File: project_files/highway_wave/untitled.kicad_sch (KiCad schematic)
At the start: 17 parts

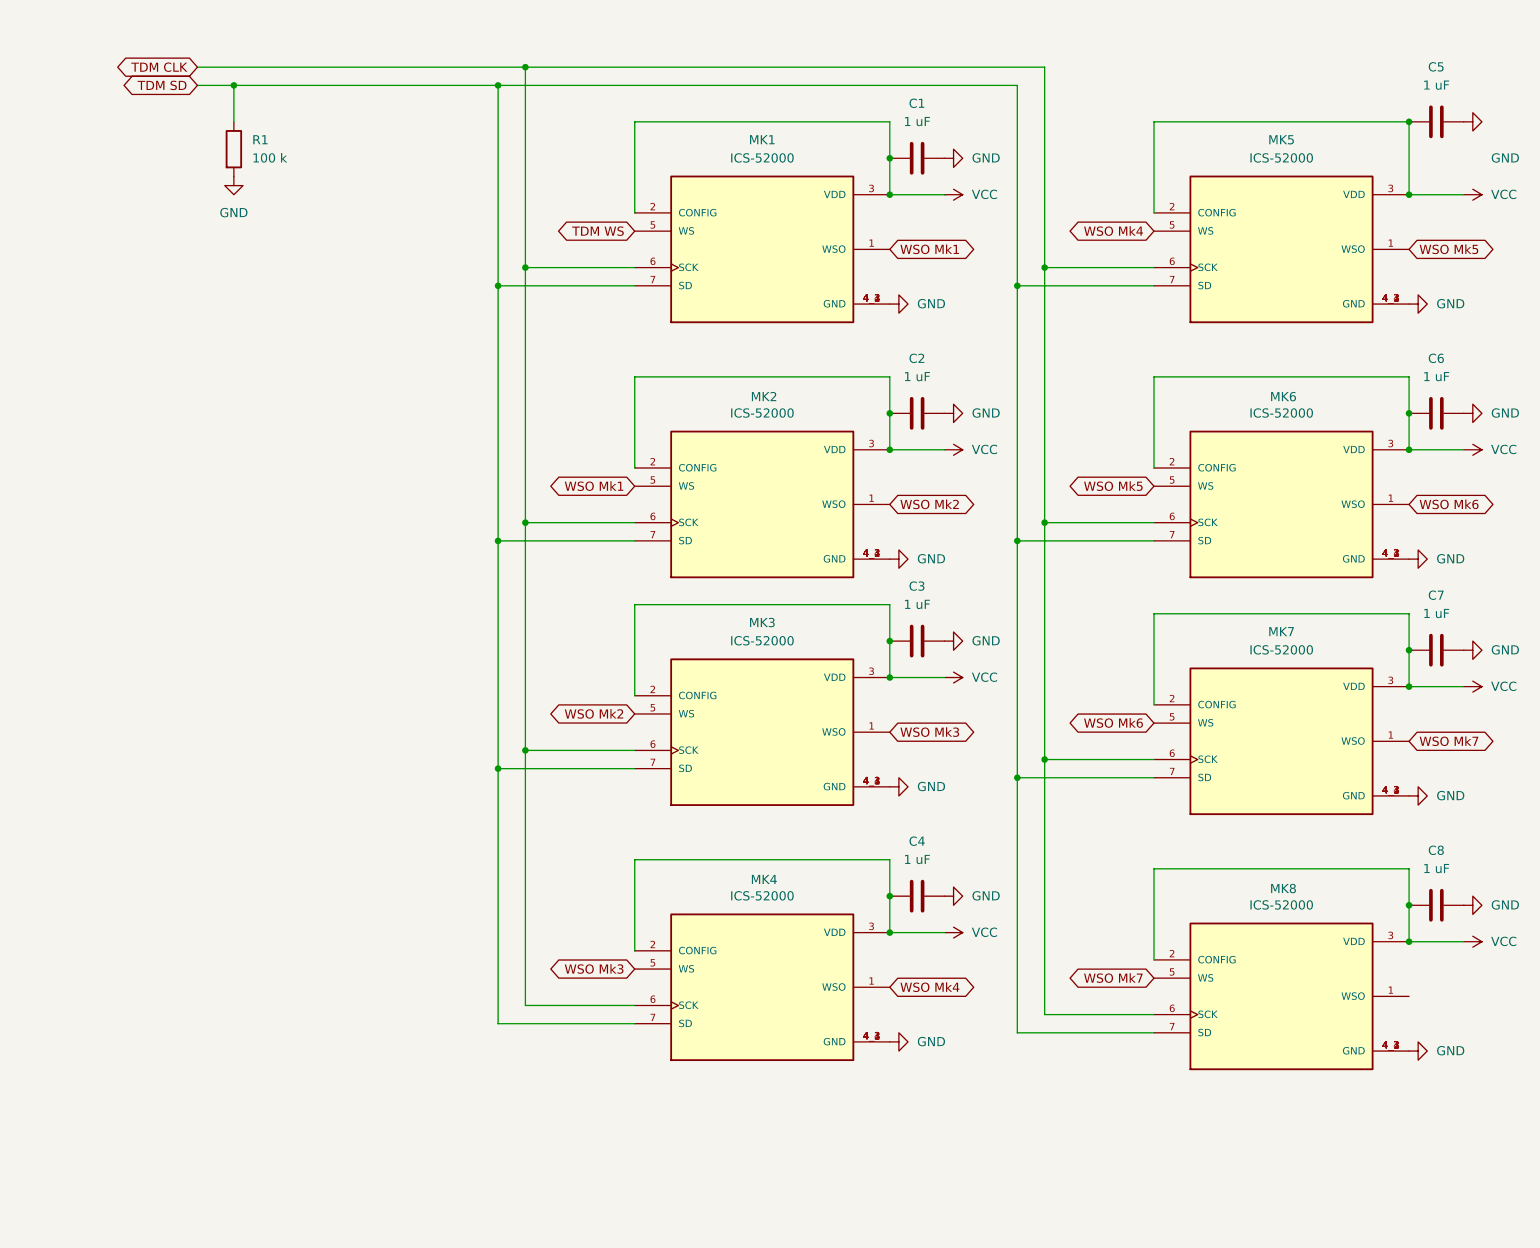
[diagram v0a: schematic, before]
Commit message: random committ
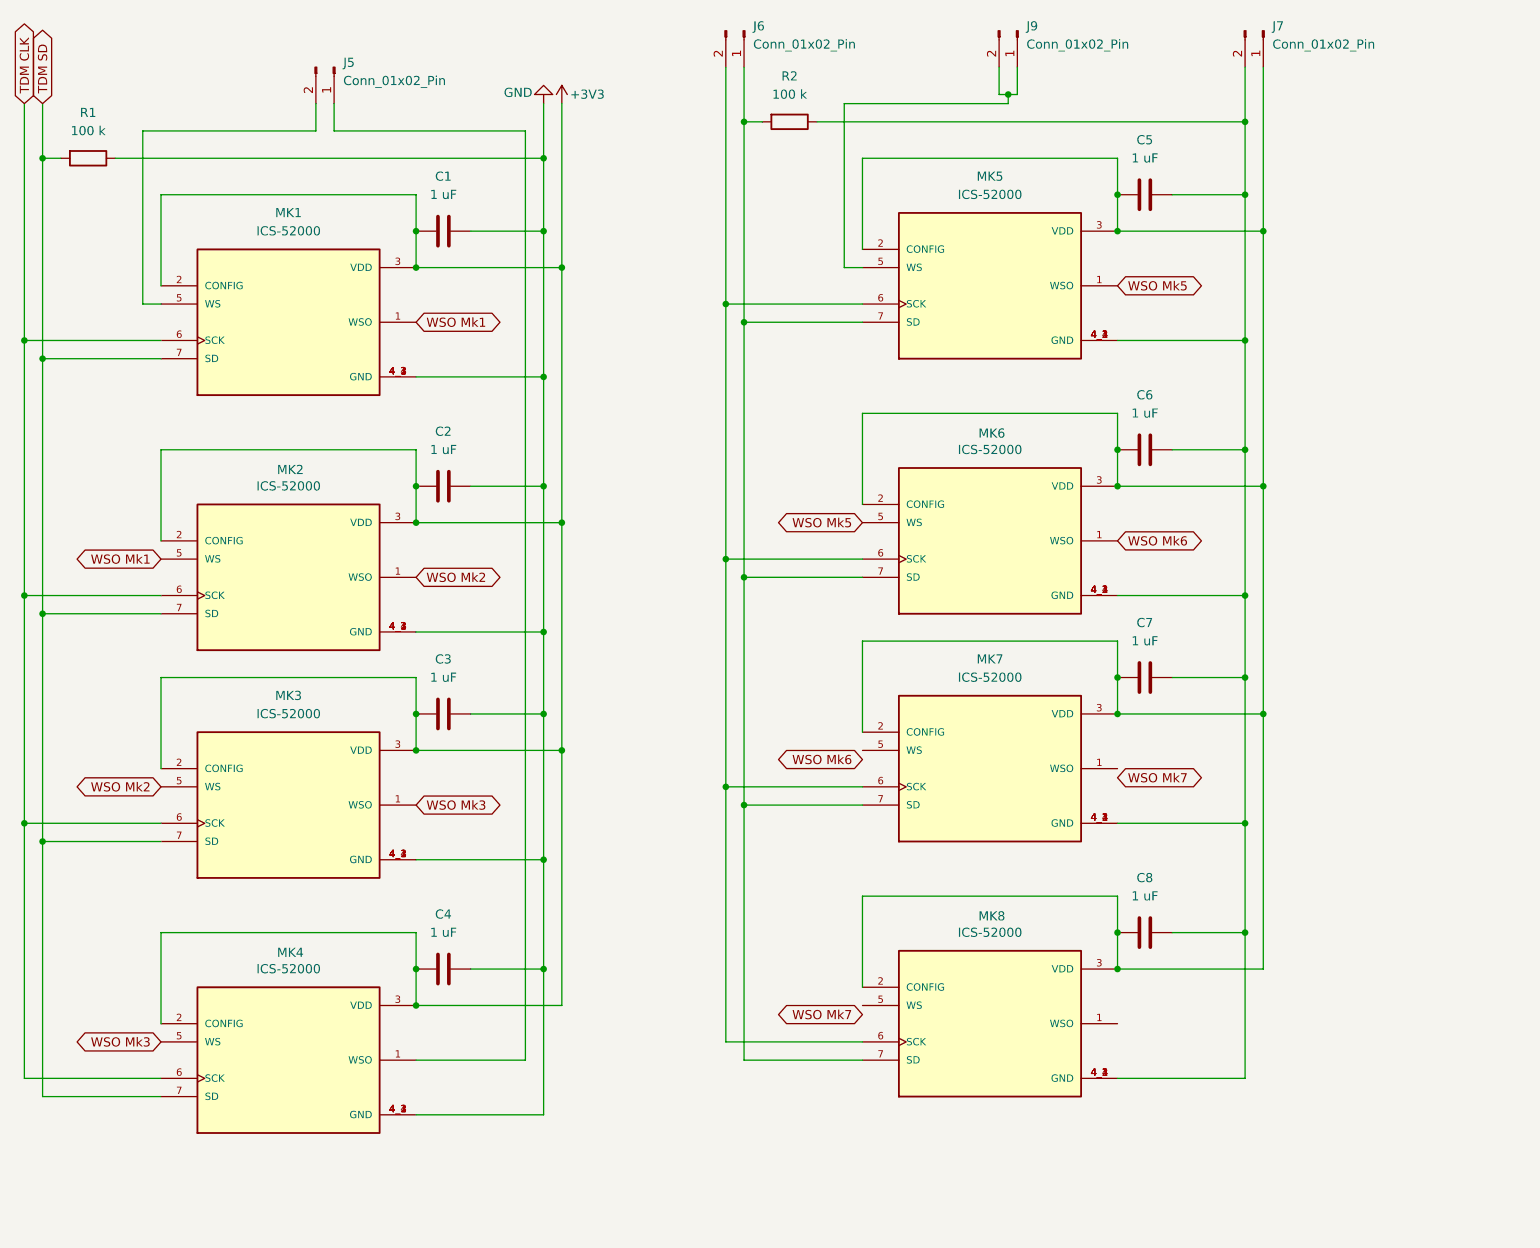
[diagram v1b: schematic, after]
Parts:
- added J5, J6, J7, J9: Conn_01x02_Pin, Connector_Phoenix_GMSTB:PhoenixContact_GMSTBVA_2,5_2-G_1x02_P7.50mm_Vertical, symbol Connector:Conn_01x02_Pin
- added R2: 100 k, Resistor_THT:R_Axial_DIN0207_L6.3mm_D2.5mm_P7.62mm_Horizontal, symbol Device:R
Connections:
- net GND: now also R1.1; no longer C5.2, C6.2, C7.2, C8.2, MK5.4_1 (GND), MK5.4_2 (GND), MK5.4_3 (GND), MK5.4_4 (GND), MK6.4_1 (GND), MK6.4_2 (GND), MK6.4_3 (GND), MK6.4_4 (GND), MK7.4_1 (GND), MK7.4_2 (GND), MK7.4_3 (GND), MK7.4_4 (GND), MK8.4_1 (GND), MK8.4_2 (GND), MK8.4_3 (GND), MK8.4_4 (GND), R1.2
- net TDM CLK: no longer MK5.6 (SCK), MK6.6 (SCK), MK7.6 (SCK), MK8.6 (SCK)
- net TDM SD: now also R1.2; no longer MK5.7 (SD), MK6.7 (SD), MK7.7 (SD), MK8.7 (SD), R1.1
- net WSO Mk6: no longer MK7.5 (WS)
- net WSO Mk7: no longer MK7.1 (WSO), MK8.5 (WS)
- net TDM WS: no longer names the net of MK1.5 (WS)
- net TDM WS: now also J5.2 (Pin_2)
- net VCC: no longer names the net of C5.1, C6.1, C7.1, C8.1, MK5.2 (CONFIG), MK5.3 (VDD), MK6.2 (CONFIG), MK6.3 (VDD), MK7.2 (CONFIG), MK7.3 (VDD), MK8.2 (CONFIG), MK8.3 (VDD)
- net VCC: now also J7.1 (Pin_1); no longer C1.1, C2.1, C3.1, C4.1, MK1.2 (CONFIG), MK1.3 (VDD), MK2.2 (CONFIG), MK2.3 (VDD), MK3.2 (CONFIG), MK3.3 (VDD), MK4.2 (CONFIG), MK4.3 (VDD)
- net WSO Mk4: no longer names the net of MK5.5 (WS)
- net WSO Mk4: now also J9.1 (Pin_1), J9.2 (Pin_2); no longer MK4.1 (WSO)
- new net: C5.2, C6.2, C7.2, C8.2, J7.2 (Pin_2), MK5.4_1 (GND), MK5.4_2 (GND), MK5.4_3 (GND), MK5.4_4 (GND), MK6.4_1 (GND), MK6.4_2 (GND), MK6.4_3 (GND), MK6.4_4 (GND), MK7.4_1 (GND), MK7.4_2 (GND), MK7.4_3 (GND), MK7.4_4 (GND), MK8.4_1 (GND), MK8.4_2 (GND), MK8.4_3 (GND), MK8.4_4 (GND), R2.1
- new net: J6.1 (Pin_1), MK5.7 (SD), MK6.7 (SD), MK7.7 (SD), MK8.7 (SD), R2.2
- new net: J6.2 (Pin_2), MK5.6 (SCK), MK6.6 (SCK), MK7.6 (SCK), MK8.6 (SCK)
- new net: J5.1 (Pin_1), MK4.1 (WSO)
- new net +3V3: C1.1, C2.1, C3.1, C4.1, MK1.2 (CONFIG), MK1.3 (VDD), MK2.2 (CONFIG), MK2.3 (VDD), MK3.2 (CONFIG), MK3.3 (VDD), MK4.2 (CONFIG), MK4.3 (VDD)
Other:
- moved on the sheet: C1, C2, C3, C4, MK1, MK2, MK3, MK4, R1

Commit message: fixed pcb
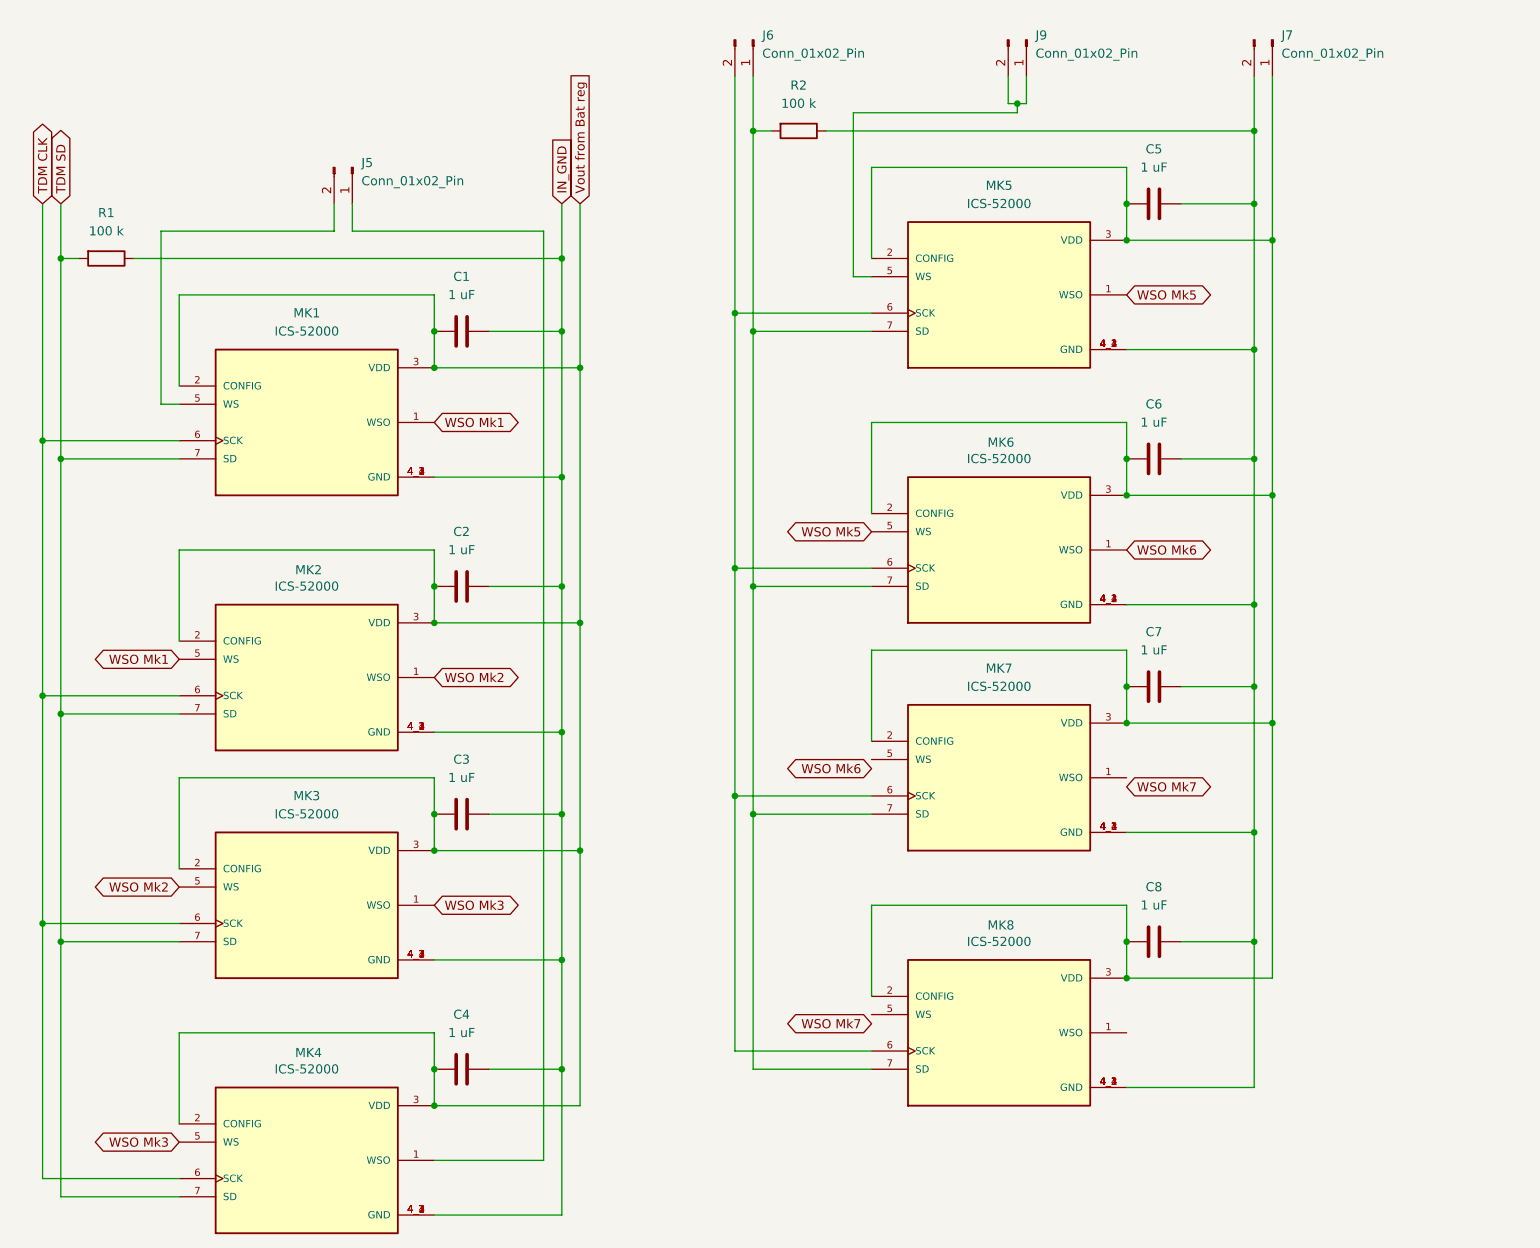
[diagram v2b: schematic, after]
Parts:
- C1, C2, C3, C4, C5, C6, C7, C8: footprint Capacitor_THT:CP_Radial_D8.0mm_P5.00mm -> Capacitor_THT:CP_Radial_D5.0mm_P2.50mm
- J5, J6, J7, J9: footprint Connector_Phoenix_GMSTB:PhoenixContact_GMSTBVA_2,5_2-G_1x02_P7.50mm_Vertical -> Connector_JST:JST_PH_B2B-PH-K_1x02_P2.00mm_Vertical
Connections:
- net +3V3 renamed Vout from Bat reg
- net GND renamed IN_GND
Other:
- moved on the sheet: C1, C2, C3, C4, C5, C6, C7, C8, J5, J6, J7, J9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
